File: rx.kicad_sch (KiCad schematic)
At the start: 32 parts, among them U1 CC1200

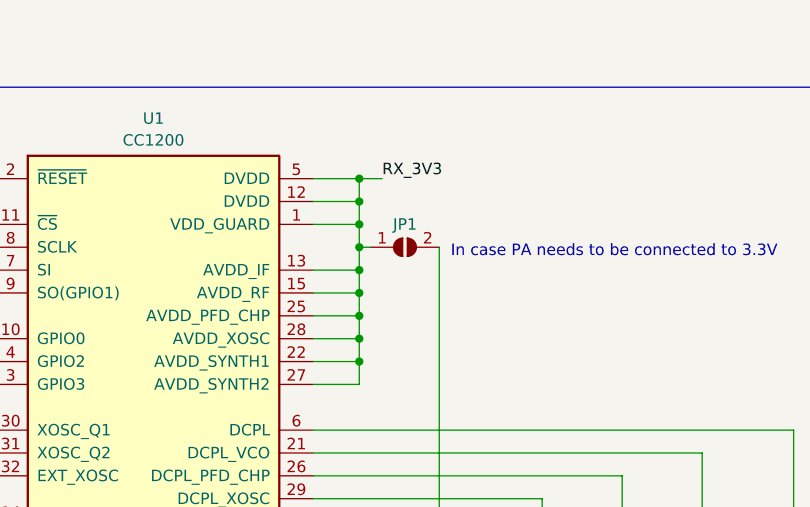
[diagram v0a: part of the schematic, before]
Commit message: PN update
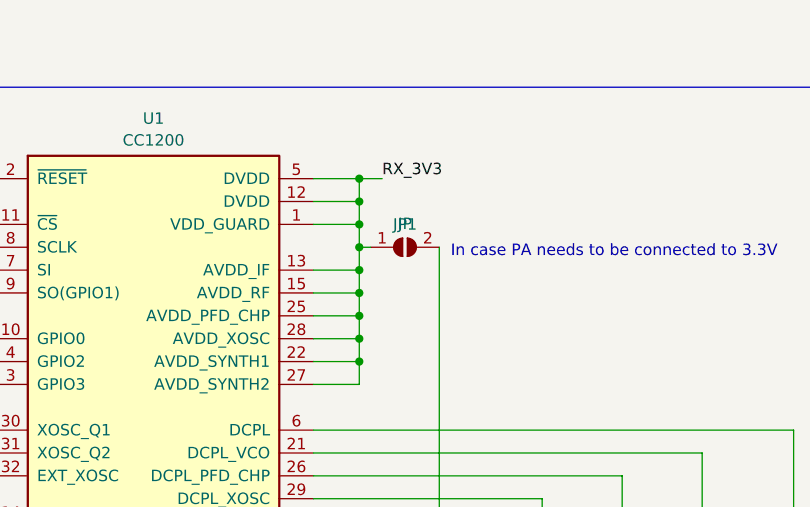
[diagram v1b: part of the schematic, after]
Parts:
- C5: PN (none) -> C0603C223K4RACTU
- C5: PN (none) -> GRM1885C1H9R1BA01D
- C5: PN (none) -> CC0603CRNPO9BN5R1
- C5: PN (none) -> GRM1885C1H6R2BA01D
- FB1: PN (none) -> BLM18KG601SH1D
- JP1: value ~ -> JP; PN (none) -> -
- U1: PN (none) -> CC1200RHBR
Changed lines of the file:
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@@
       (effects (font (size 1.27 1.27)) hide)
     )
-    (property "PN" "" (at 247.65 101.6 0)
+    (property "PN" "C0603C223K4RACTU" (at 247.65 101.6 0)
       (effects (font (size 1.27 1.27)) hide)
     )
@@
       (effects (font (size 1.27 1.27)))
     )
-    (property "Value" "~" (at 204.47 65.9709 0)
+    (property "Value" "JP" (at 204.47 65.9709 0)
       (effects (font (size 1.27 1.27)))
     )
@@
       (effects (font (size 1.27 1.27)) hide)
     )
+    (property "PN" "-" (at 204.47 68.58 0)
+      (effects (font (size 1.27 1.27)) hide)
+    )
     (pin "1")
     (pin "2")
@@
       (effects (font (size 1.27 1.27)) hide)
     )
-    (property "PN" "" (at 152.4 93.98 0)
+    (property "PN" "GRM1885C1H9R1BA01D" (at 152.4 93.98 0)
       (effects (font (size 1.27 1.27)) hide)
     )
@@
       (effects (font (size 1.27 1.27)) hide)
     )
+    (property "PN" "CC0603CRNPO9BN5R1" (at 203.2 128.27 0)
+      (effects (font (size 1.27 1.27)) hide)
+    )
     (pin "1")
     (pin "2")
@@
       (effects (font (size 1.27 1.27)) hide)
     )
+    (property "PN" "CC0603CRNPO9BN5R1" (at 219.71 127 0)
+      (effects (font (size 1.27 1.27)) hide)
+    )
     (pin "1")
     (pin "2")
@@
       (effects (font (size 1.27 1.27)) hide)
     )
+    (property "PN" "CC0603CRNPO9BN5R1" (at 237.49 134.62 0)
+      (effects (font (size 1.27 1.27)) hide)
+    )
     (pin "1")
     (pin "2")
@@
       (effects (font (size 1.27 1.27)) hide)
     )
+    (property "PN" "GRM1885C1H6R2BA01D" (at 242.57 139.7 0)
+      (effects (font (size 1.27 1.27)) hide)
+    )
     (pin "1")
     (pin "2")
@@
     )
     (property "Datasheet" "http://www.ti.com/lit/ds/symlink/cc1200.pdf" (at 163.83 57.15 0)
+      (effects (font (size 1.27 1.27)) hide)
+    )
+    (property "PN" "CC1200RHBR" (at 176.53 86.36 0)
       (effects (font (size 1.27 1.27)) hide)
     )
@@
       (effects (font (size 1.27 1.27)) hide)
     )
-    (property "PN" "" (at 201.93 200.66 90)
-      (effects (font (size 1.27 1.27)) hide)
-    )
+    (property "PN" "BLM18KG601SH1D" (at 201.93 200.66 90)
+      (effects (font (size 1.27 1.27)) hide)
+    )
